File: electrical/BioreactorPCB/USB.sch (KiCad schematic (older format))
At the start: 7 parts, among them J10 USB_B, U2 FT232RL

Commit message: added missing electrolytic capacitors for A4988 breakouts. Preliminary layout now in place
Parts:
- C3: footprint Capacitor_THT:CP_Radial_Tantal_D5.0mm_P2.50mm -> Capacitor_THT:C_Disc_D5.0mm_W2.5mm_P2.50mm
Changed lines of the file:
@@
 F 0 "C3" V 5873 2750 50  0000 C CNN
 F 1 ".1 uF" V 5964 2750 50  0000 C CNN
-F 2 "Capacitor_THT:CP_Radial_Tantal_D5.0mm_P2.50mm" H 6163 2600 50  0001 C CNN
+F 2 "Capacitor_THT:C_Disc_D5.0mm_W2.5mm_P2.50mm" H 6163 2600 50  0001 C CNN
 F 3 "~" H 6125 2750 50  0001 C CNN
 	1    6125 2750

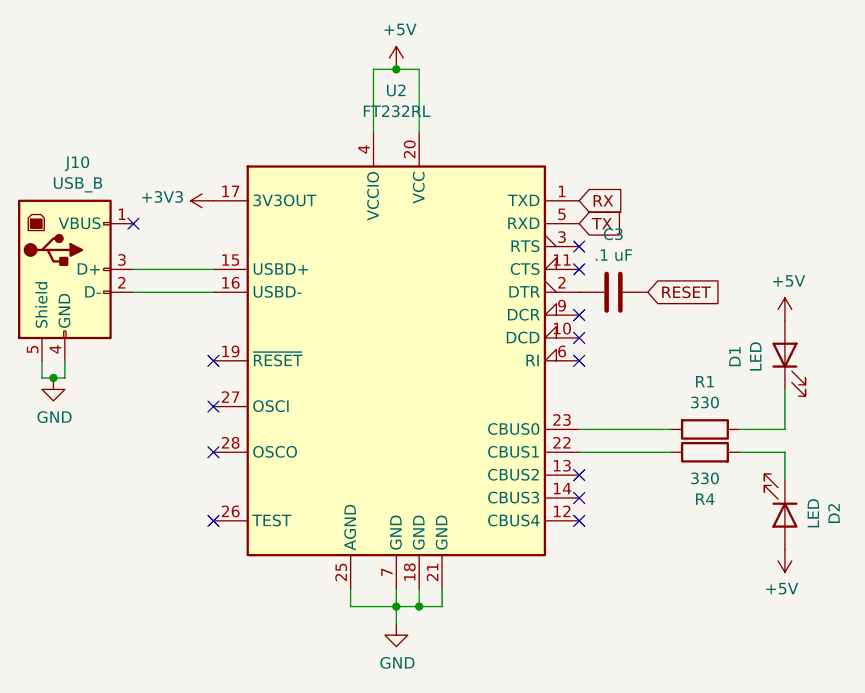
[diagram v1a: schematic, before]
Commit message: motherboard layout complete.
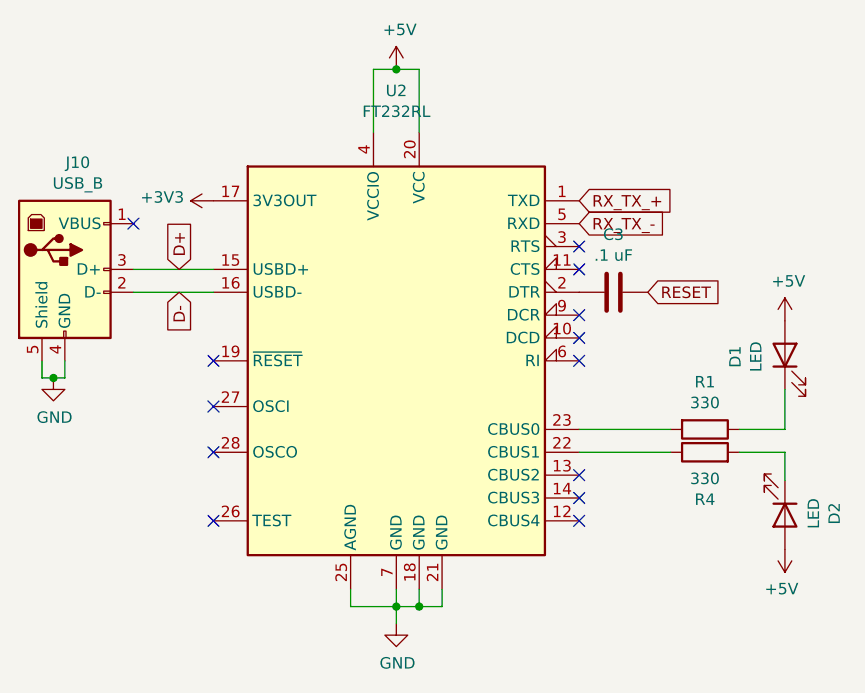
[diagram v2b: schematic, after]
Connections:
- net D+: now reaches J10.3 (D+), U2.15 (USBD+)
- net D-: now reaches J10.2 (D-), U2.16 (USBD-)
- net RX renamed RX_TX_+
- net TX renamed RX_TX_-
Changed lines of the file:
@@
 RESET
 Text GLabel 5975 2350 2    50   Input ~ 0
-RX
+RX_TX_+
 Text GLabel 5975 2450 2    50   Input ~ 0
-TX
+RX_TX_-
 $Comp
 L power:+5V #PWR?
@@
 	1    0    0    -1
 $EndComp
+Text GLabel 4225 2650 1    50   Input ~ 0
+D+
+Text GLabel 4225 2750 3    50   Input ~ 0
+D-
 $EndSCHEMATC

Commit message: Converted all nonpolarized resistors and capacitors to SMD. USB now has differential pairs that conform to design guidelines. Lots of traces, to what end? idk.
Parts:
- C3: footprint Capacitor_THT:C_Disc_D5.0mm_W2.5mm_P2.50mm -> Capacitor_SMD:C_0603_1608Metric_Pad1.08x0.95mm_HandSolder
- R1, R4: footprint Resistor_THT:R_Axial_DIN0204_L3.6mm_D1.6mm_P5.08mm_Horizontal -> Resistor_SMD:R_0805_2012Metric_Pad1.20x1.40mm_HandSolder
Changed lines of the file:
@@
 F 0 "C3" V 5873 2750 50  0000 C CNN
 F 1 ".1 uF" V 5964 2750 50  0000 C CNN
-F 2 "Capacitor_THT:C_Disc_D5.0mm_W2.5mm_P2.50mm" H 6163 2600 50  0001 C CNN
+F 2 "Capacitor_SMD:C_0603_1608Metric_Pad1.08x0.95mm_HandSolder" H 6163 2600 50  0001 C CNN
 F 3 "~" H 6125 2750 50  0001 C CNN
 	1    6125 2750
@@
 F 0 "R4" V 6318 3450 50  0000 C CNN
 F 1 "330" V 6409 3450 50  0000 C CNN
-F 2 "Resistor_THT:R_Axial_DIN0204_L3.6mm_D1.6mm_P5.08mm_Horizontal" V 6455 3450 50  0001 C CNN
+F 2 "Resistor_SMD:R_0805_2012Metric_Pad1.20x1.40mm_HandSolder" V 6455 3450 50  0001 C CNN
 F 3 "~" H 6525 3450 50  0001 C CNN
 	1    6525 3450
@@
 F 0 "R1" V 6318 3350 50  0000 C CNN
 F 1 "330" V 6409 3350 50  0000 C CNN
-F 2 "Resistor_THT:R_Axial_DIN0204_L3.6mm_D1.6mm_P5.08mm_Horizontal" V 6455 3350 50  0001 C CNN
+F 2 "Resistor_SMD:R_0805_2012Metric_Pad1.20x1.40mm_HandSolder" V 6455 3350 50  0001 C CNN
 F 3 "~" H 6525 3350 50  0001 C CNN
 	1    6525 3350
